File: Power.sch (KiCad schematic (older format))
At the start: 80 parts, among them J3 USB, J4 OTG, Q1 DTA114YKA, SW3 RST, U1 AllWinner-S3(FBGA-234), U3 AXP209(QFN-48), U4 SY8089AAAC, U5 SY6280AAC

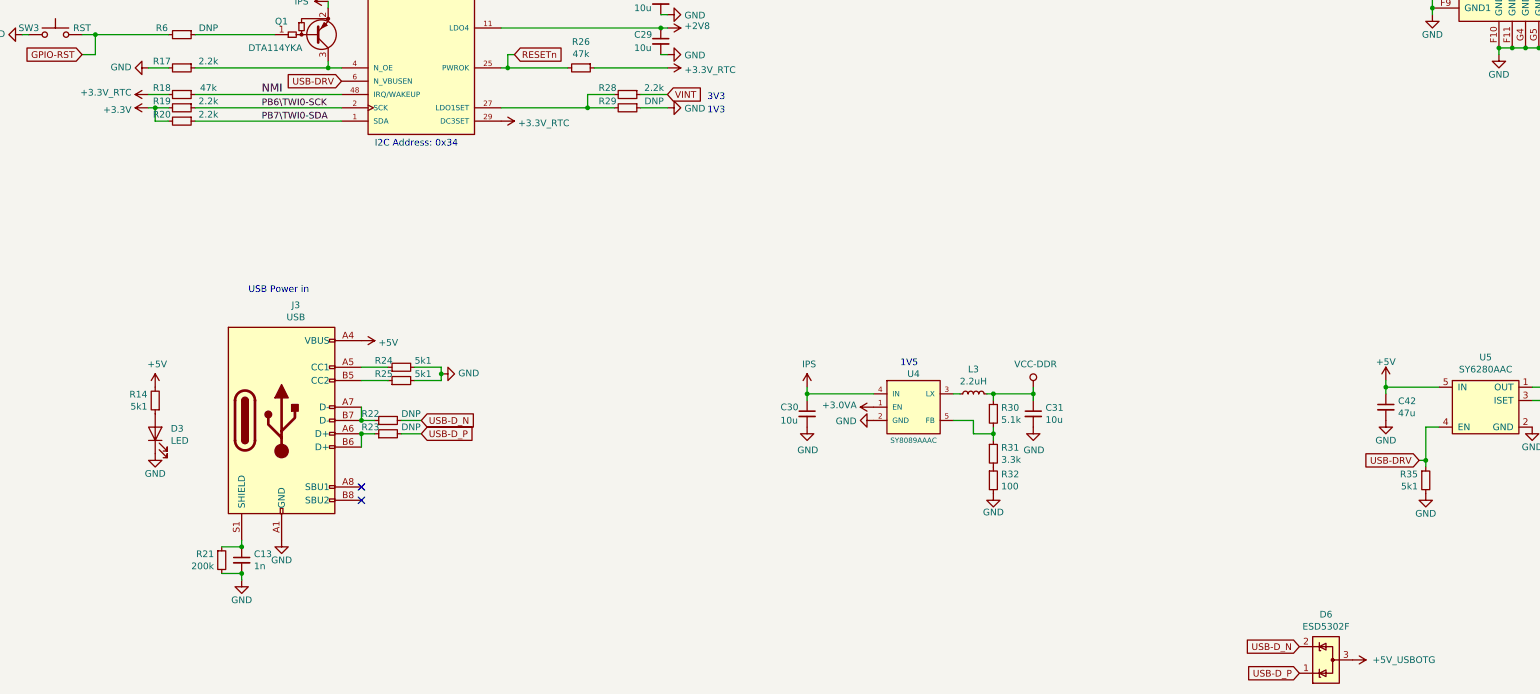
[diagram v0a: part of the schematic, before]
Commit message: added i2c to axp209, fixed tvs diodes
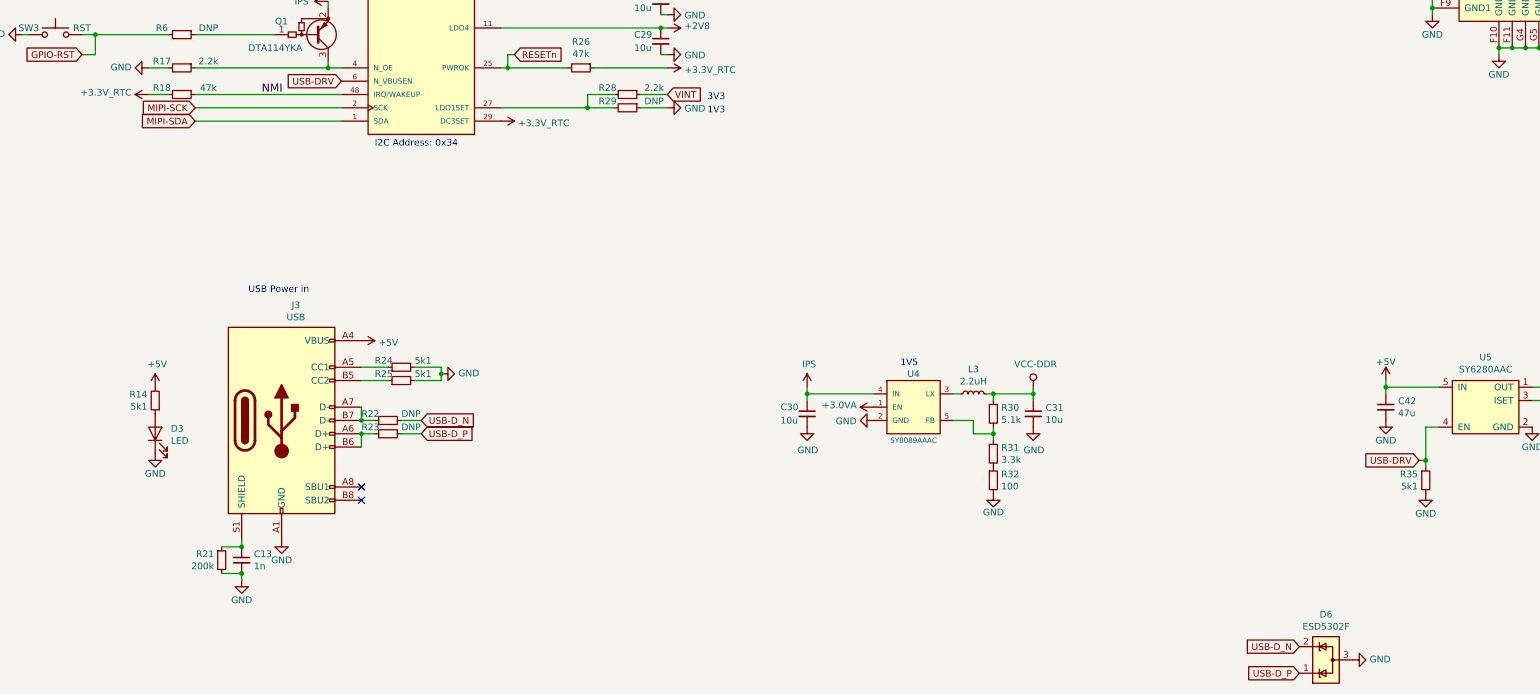
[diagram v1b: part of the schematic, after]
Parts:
- removed R19, R20: 2.2k, otter:R_0402, symbol Device:R_Small
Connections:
- net +5V_USBOTG: no longer D6.3 (A)
- net GND: now also D6.3 (A)
- net PB6\TWI0-SCK renamed MIPI-SCK
- net PB7\TWI0-SDA renamed MIPI-SDA
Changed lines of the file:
@@
 Text Notes 6000 5900 0    50   ~ 0
 1V3\n
-Text Label 2650 5850 0    50   ~ 0
-PB6\TWI0-SCK
-Text Label 2650 5950 0    50   ~ 0
-PB7\TWI0-SDA
-$Comp
-L Device:R_Small R?
-U 1 1 65EC7F5C
-P 2050 5850
-AR Path="/65EC7F5C" Ref="R?"  Part="1"
-AR Path="/602ACDF9/65EC7F5C" Ref="R19"  Part="1"
-F 0 "R19" V 2000 5700 50  0000 C CNN
-F 1 "2.2k" V 2000 6050 50  0000 C CNN
-F 2 "otter:R_0402" H 2050 5850 50  0001 C CNN
-F 3 "~" H 2050 5850 50  0001 C CNN
-	1    2050 5850
-	0    1    1    0
-$EndComp
-$Comp
-L Device:R_Small R?
-U 1 1 65EEA2F4
-P 2050 5950
-AR Path="/65EEA2F4" Ref="R?"  Part="1"
-AR Path="/602ACDF9/65EEA2F4" Ref="R20"  Part="1"
-F 0 "R20" V 2000 5800 50  0000 C CNN
-F 1 "2.2k" V 2000 6150 50  0000 C CNN
-F 2 "otter:R_0402" H 2050 5950 50  0001 C CNN
-F 3 "~" H 2050 5950 50  0001 C CNN
-	1    2050 5950
-	0    1    1    0
-$EndComp
-$Comp
-L S3-OLinuXino_Rev_A:+3.3V #PWR?
-U 1 1 65F75DFC
-P 1800 5850
-AR Path="/5D8A1FAC/65F75DFC" Ref="#PWR?"  Part="1"
-AR Path="/65F75DFC" Ref="#PWR?"  Part="1"
-AR Path="/602ACDF9/65F75DFC" Ref="#PWR0163"  Part="1"
-F 0 "#PWR0163" H 1800 5700 50  0001 C CNN
-F 1 "+3.3V" V 1815 5978 50  0000 L CNN
-F 2 "" H 1800 5850 60  0000 C CNN
-F 3 "" H 1800 5850 60  0000 C CNN
-	1    1800 5850
-	0    -1   1    0
-$EndComp
-Wire Wire Line
-	1950 5850 1850 5850
-Wire Wire Line
-	1850 5850 1850 5950
-Wire Wire Line
-	1850 5950 1950 5950
-Wire Wire Line
-	1850 5850 1800 5850
-Connection ~ 1850 5850
 Wire Wire Line
 	2150 5850 3250 5850
@@
 	0    -1   -1   0
 $EndComp
-$Comp
-L S3-OLinuXino_Rev_A:+5V_USBOTG #PWR?
-U 1 1 5FC176D0
-P 10850 10000
-AR Path="/5D8A1FAC/5FC176D0" Ref="#PWR?"  Part="1"
-AR Path="/5FC176D0" Ref="#PWR?"  Part="1"
-AR Path="/602ACDF9/5FC176D0" Ref="#PWR0110"  Part="1"
-F 0 "#PWR0110" H 10850 9850 50  0001 C CNN
-F 1 "+5V_USBOTG" V 10850 10150 50  0000 L CNN
-F 2 "" H 10850 10000 60  0000 C CNN
-F 3 "" H 10850 10000 60  0000 C CNN
-	1    10850 10000
-	0    1    1    0
-$EndComp
 Connection ~ 3400 8300
 Connection ~ 3400 8200
@@
 	1950 5300 1400 5300
 Connection ~ 1400 5300
+$Comp
+L otter:GND #PWR?
+U 1 1 6036508A
+P 10850 10000
+AR Path="/6036508A" Ref="#PWR?"  Part="1"
+AR Path="/602ACDF9/6036508A" Ref="#PWR0115"  Part="1"
+F 0 "#PWR0115" H 10850 9750 50  0001 C CNN
+F 1 "GND" V 10855 9872 50  0000 R CNN
+F 2 "" H 10850 10000 60  0000 C CNN
+F 3 "" H 10850 10000 60  0000 C CNN
+	1    10850 10000
+	0    -1   -1   0
+$EndComp
+Text GLabel 2150 5950 0    50   Input ~ 0
+MIPI-SDA
+Text GLabel 2150 5850 0    50   Input ~ 0
+MIPI-SCK
 $EndSCHEMATC
